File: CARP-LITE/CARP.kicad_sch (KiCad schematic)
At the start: 111 parts, among them J1 USB-C, J10 PYRO_2, J3 I2C1+3V3, J4 2S XT30, J5 UART+5V+I2C1, J6 PYRO_1, J8 PWM1+6V, J9 PWM2+6V, Q5 SQ2318CES, Q6 SQ2318CES, Q7 SQ2318CES, SW1 SW_Push, SW2 SW_Push, U1 W25Q128JVSIMTR (16MB), U10 TPS62130A, U2 W25Q32RVXHJQ (2MB), U3 3V3 LDO, U4 RP2350_60QFN, U5 LSM6DSO, U6 BMP390, U7 5V LDO, U8 6V LDO, Y1 ABM8-272-T3

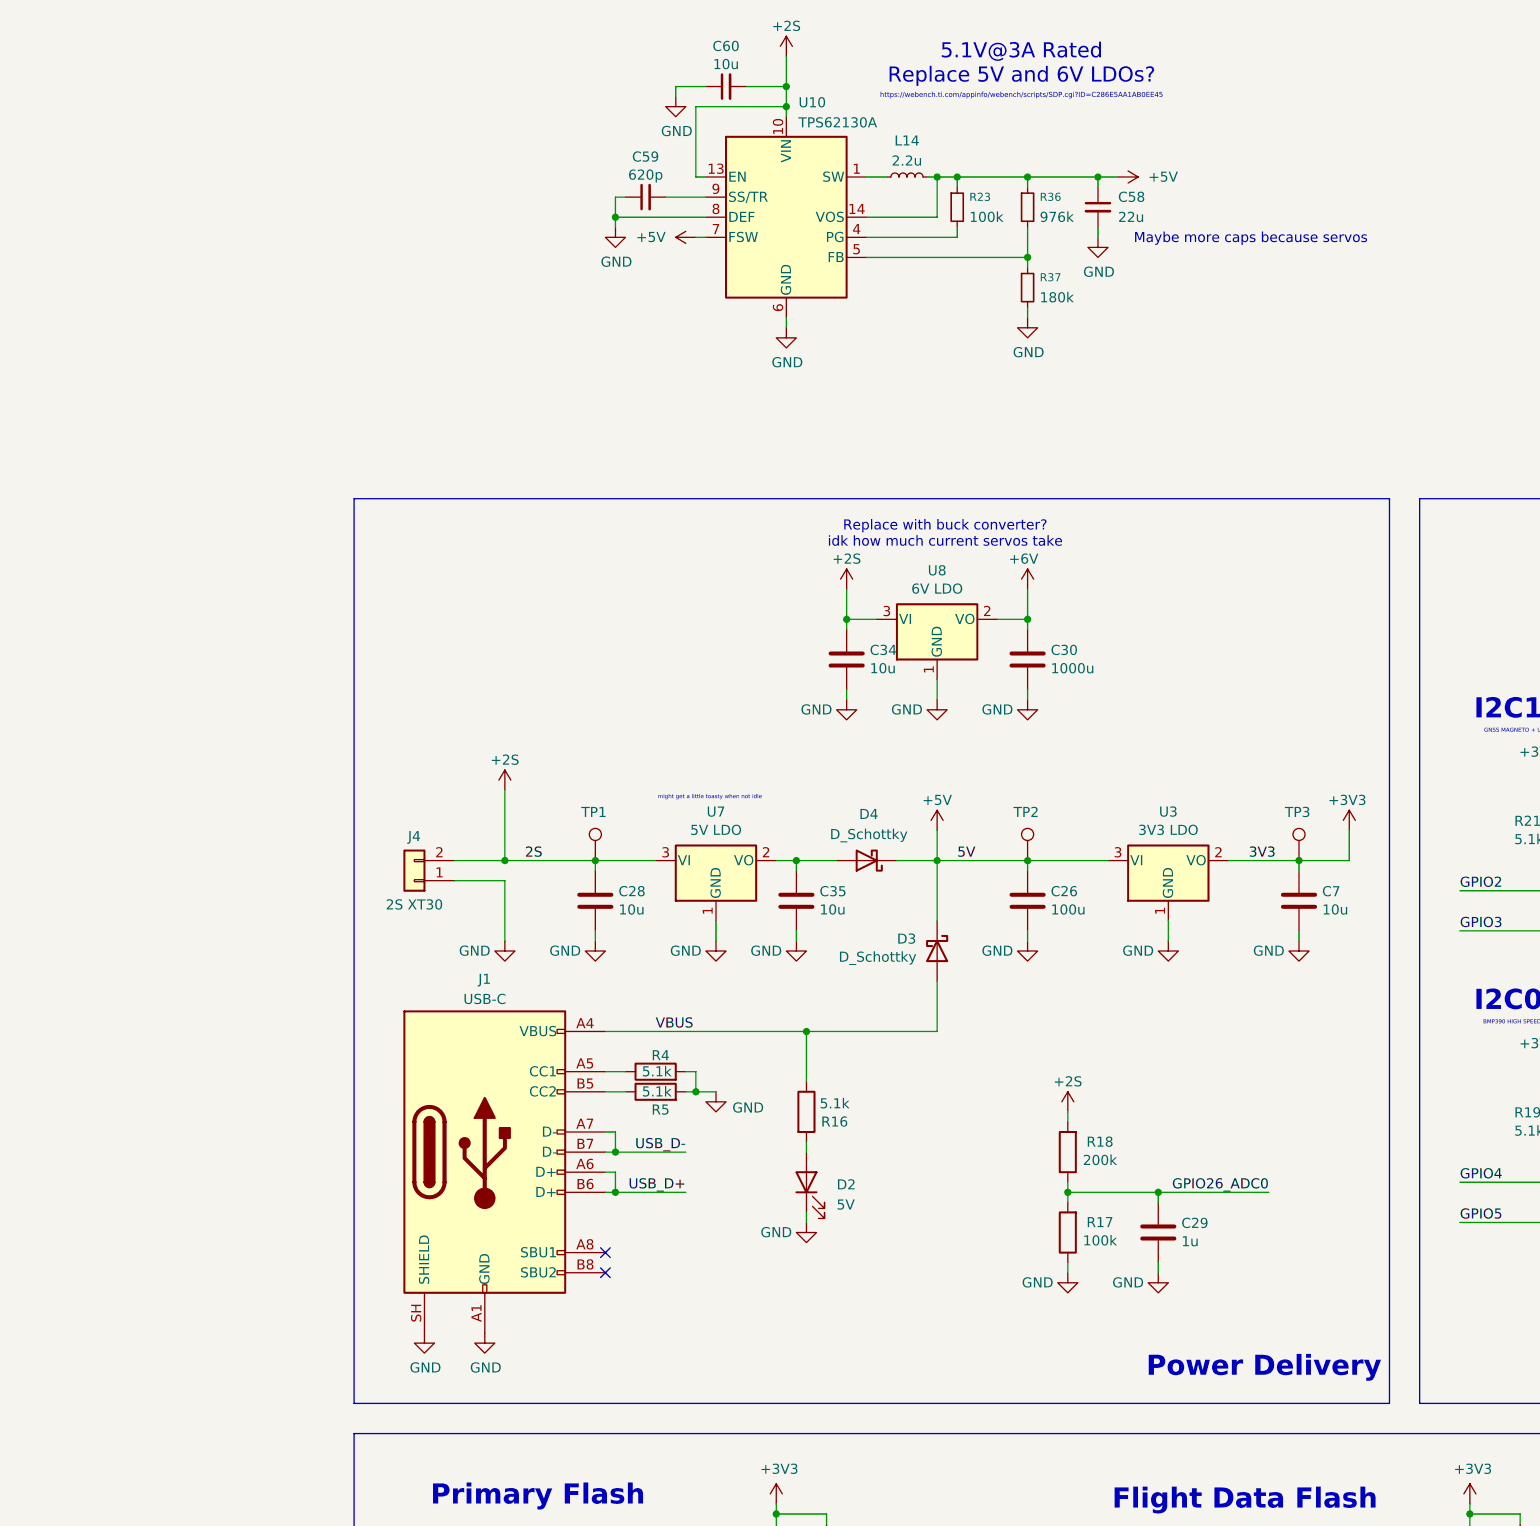
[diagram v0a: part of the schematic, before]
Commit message: power delivery revamp
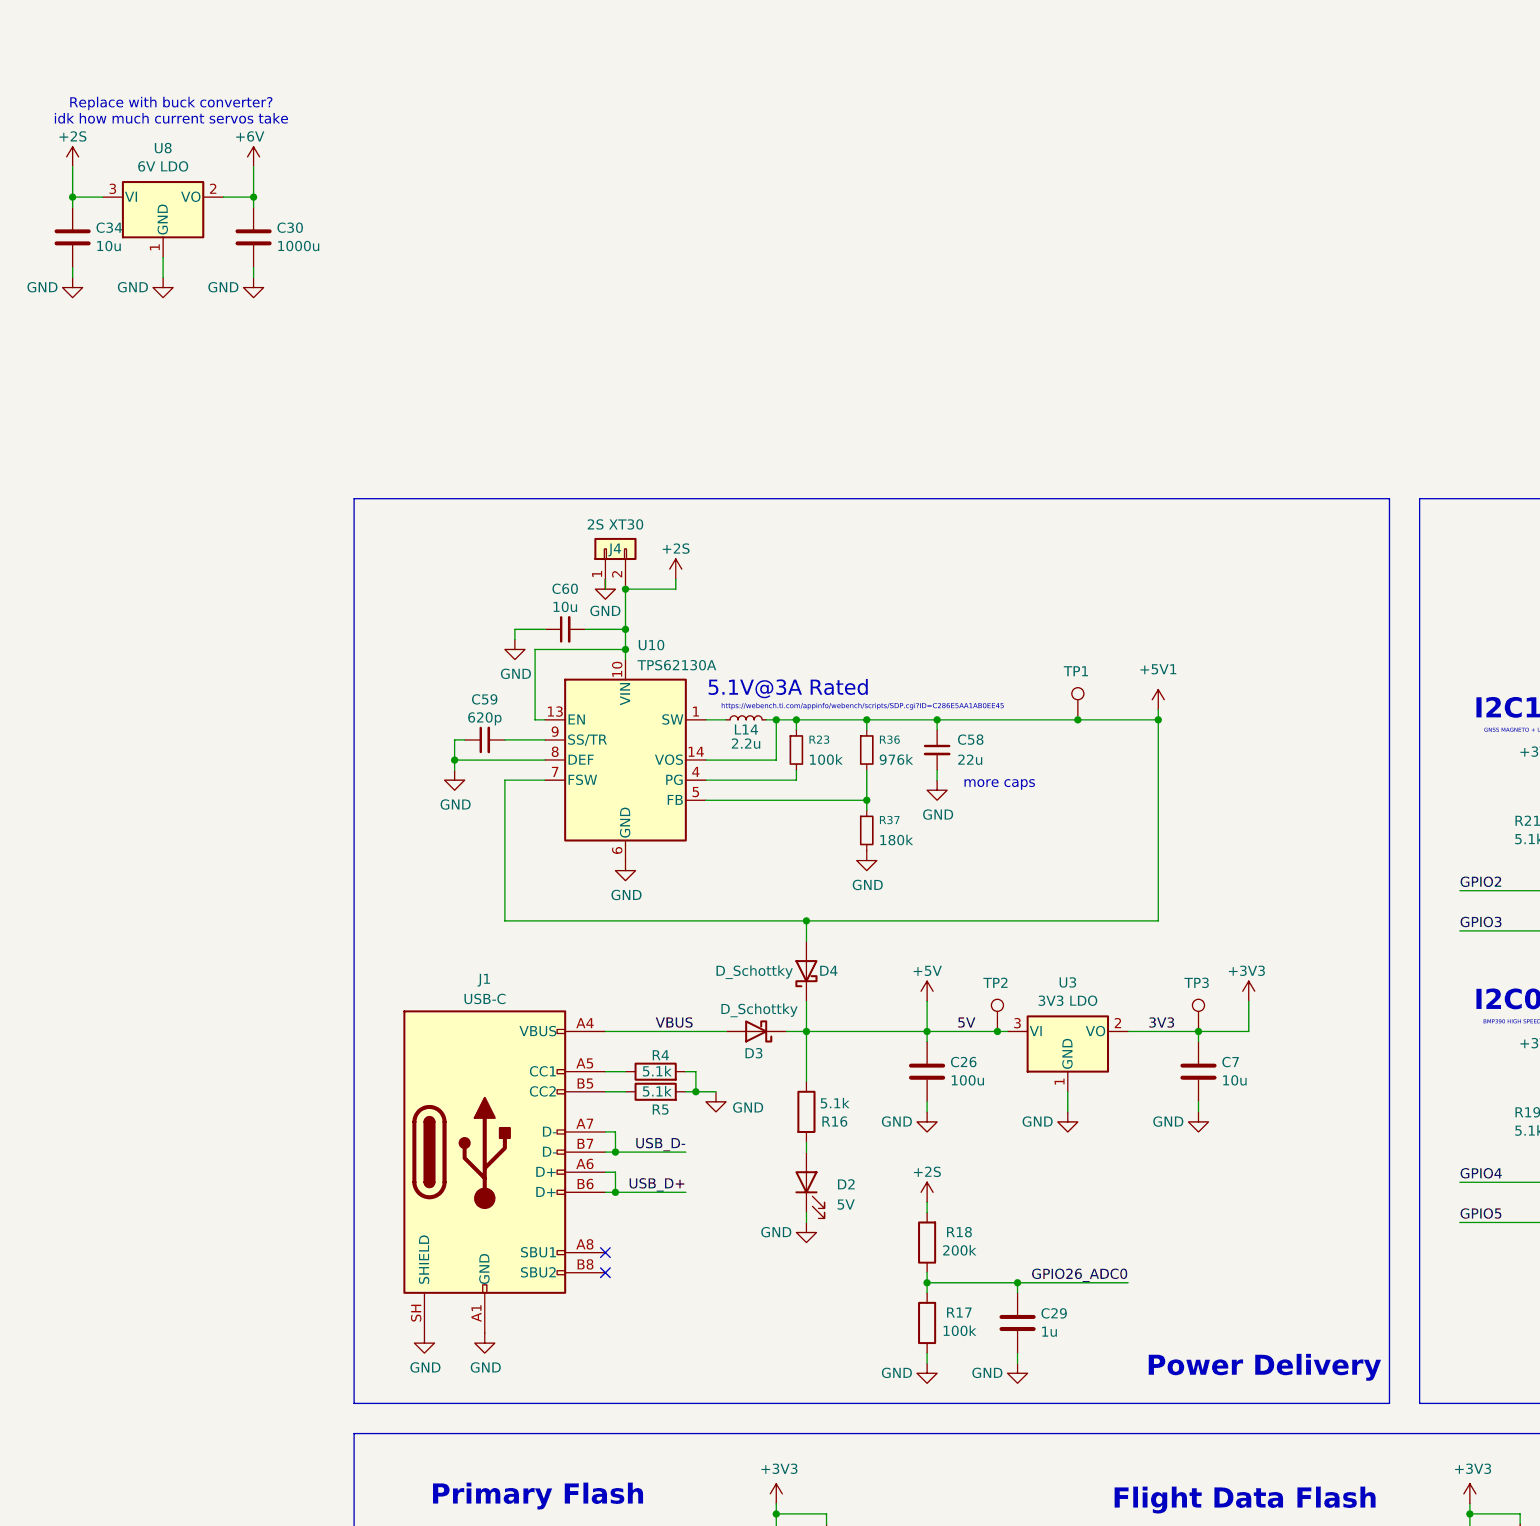
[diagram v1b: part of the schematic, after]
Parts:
- removed C28, C35: 10u, Capacitor_SMD:C_0603_1608Metric, symbol Device:C
- removed U7: 5V LDO, Package_TO_SOT_SMD:SOT-223-3_TabPin2, symbol Regulator_Linear:NCP1117-3.3_SOT223
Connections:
- net +2S: no longer TP1.1
- net +5V: now also R16.1; no longer C58.1, L14.2, R23.1, R36.1, U10.14 (VOS), U10.7 (FSW)
- net VBUS: no longer R16.1
- net +5V1: now reaches D4.2 (A)
- net +5V1: now also C58.1, L14.2, R23.1, R36.1, TP1.1, U10.14 (VOS), U10.7 (FSW)
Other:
- note added: "5.1V@3A Rated"
- note added: "more caps"
- note removed: "5.1V@3A Rated Replace 5V and 6V LDOs?"
- note removed: "Maybe more caps because servos"
- note removed: "might get a little toasty when not idle"
- moved on the sheet: C26, C29, C30, C34, C58, C59, C60, C7, J4, L14, R17, R18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
